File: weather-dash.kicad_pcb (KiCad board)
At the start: 11 copper layers, 59.5 x 43.5 mm, 7 parts, among them J1 Conn_01x02_Pin, J3 Conn_01x03_Socket, SW1 SW_Push, U1 WEMOS_C3_Mini, U2 TFT_ST7735_SD

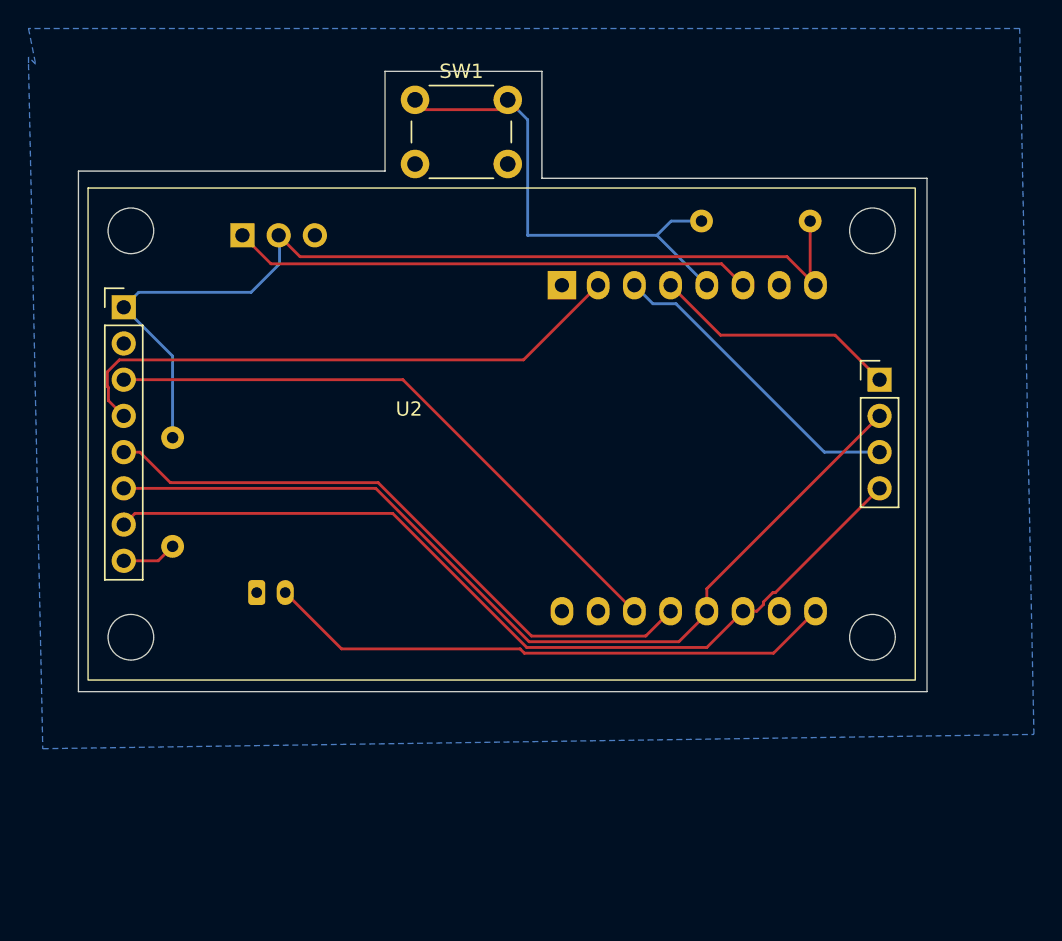
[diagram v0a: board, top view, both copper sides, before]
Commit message: updates
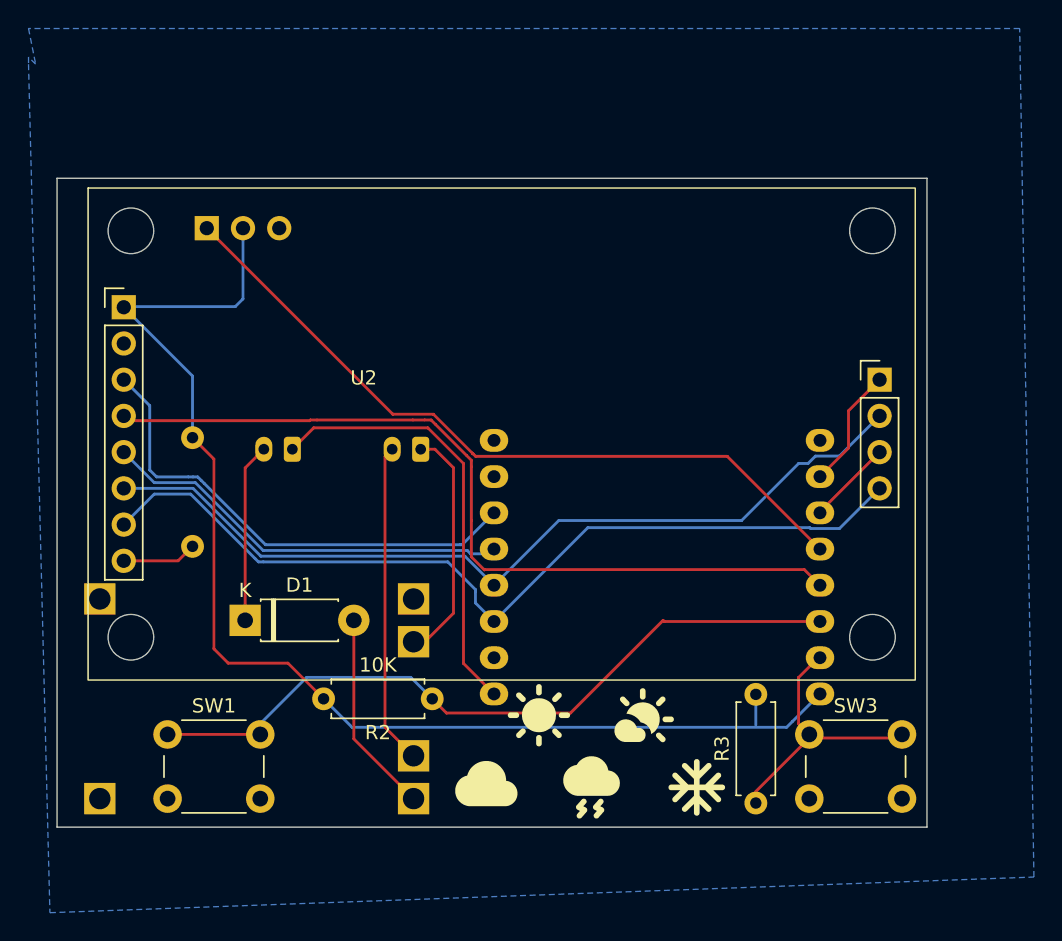
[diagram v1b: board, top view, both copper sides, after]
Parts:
- added D1: 1N5817, Diode_THT:D_DO-41_SOD81_P7.62mm_Horizontal, F.Cu at (28.2, 54.5)
- added G***: LOGO, LOGO, B.Cu at (62.5, 30.5)
- added R3: 10K, Resistor_THT:R_Axial_DIN0207_L6.3mm_D2.5mm_P7.62mm_Horizontal, F.Cu at (64.0, 67.3)
- added SW2: SW_SPDT, Connector_JST:JST_PH_B2B-PH-K_1x02_P2.00mm_Vertical, B.Cu at (31.5, 42.5)
- added SW3: SW_Push, Button_Switch_THT:SW_PUSH_6mm_H4.3mm, F.Cu at (67.8, 62.5)
- added U3: ~, asylum-weather:TP4056, B.Cu at (29.5, 60.0)
- J3: footprint Connector_PinSocket_2.54mm:PinSocket_1x03_P2.54mm_Vertical -> asylum-weather:DHT11
- R2: moved to F.Cu
- U1: footprint Module:WEMOS_D1_mini_light -> asylum-weather:WEMOS_C3_mini
- moved SW1 47.8 mm to (22.8, 62.5)
- moved R2 38.5 mm to (41.3, 60.0), turned to 180 degrees
- moved U1 19.6 mm to (57.1, 49.4), turned to 180 degrees
- moved J1 15.3 mm to (40.5, 42.5), turned to 180 degrees
- moved J3 2.55 mm to (25.5, 27.0)
- moved R1 1.40 mm to (24.5, 41.7)
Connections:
- J1 pad 1: GND -> BAT-
- J1 pad 2: VBUS -> BAT+
- R2 pad 1: BTN -> BTN1
- SW1 pad 1: BTN -> BTN1
- U1 pad 2: TFT_EN -> SD_CS
- U1 pad 4: SD_CS -> DHT11
- U1 pad 5: BTN -> TFT_EN
- U1 pad 6: DHT11 -> BTN1
- U1 pad 7: unconnected-(U1-IO5-Pad7) -> BTN2
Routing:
- net BTN1: track 0.00 -> 51.6 mm
- net BTN: track 35.7 -> 0.00 mm
- net BAT+: track 0.00 -> 22.5 mm
- net +3.3V: track 68.5 -> 88.0 mm
- net BTN2: track 0.00 -> 19.0 mm
- net TFT_EN: track 40.5 -> 57.8 mm
- net BAT-: track 0.00 -> 16.7 mm
- net MISO: track 22.0 -> 5.99 mm
- net DHT11: track 36.6 -> 52.4 mm
- net TFT_DC: track 44.4 -> 29.1 mm
- net Net-(D1-A): track 0.00 -> 14.2 mm
- net Net-(D1-K): track 0.00 -> 12.5 mm
- net VBUS: track 40.2 -> 30.7 mm
- net SD_CS: track 17.4 -> 8.53 mm
- net TFT_CS: track 42.5 -> 34.3 mm
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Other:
- board size 59.5 x 43.5 mm -> 61 x 45.5 mm
- board text added: "@grimsteel"
- board text added: "Weather Dash"
- board text added: "v0.2"
- board text removed: "BAT"
